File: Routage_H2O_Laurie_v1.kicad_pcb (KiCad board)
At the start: 2 copper layers, 110 x 100 mm, 54 parts, among them J2 Conn_01x02, J3 Conn_01x03, Q1 2N2907, Q10 TIP32, Q11 BD138, Q12 TIP31, Q13 2N2222, Q2 2N2907, Q3 2N2907, Q4 2N2222, Q5 2N2222, Q6 2N2907, Q7 2N2907, Q8 BD139, Q9 BD139, U1 Relay_1CT, U2 Jack_Mono

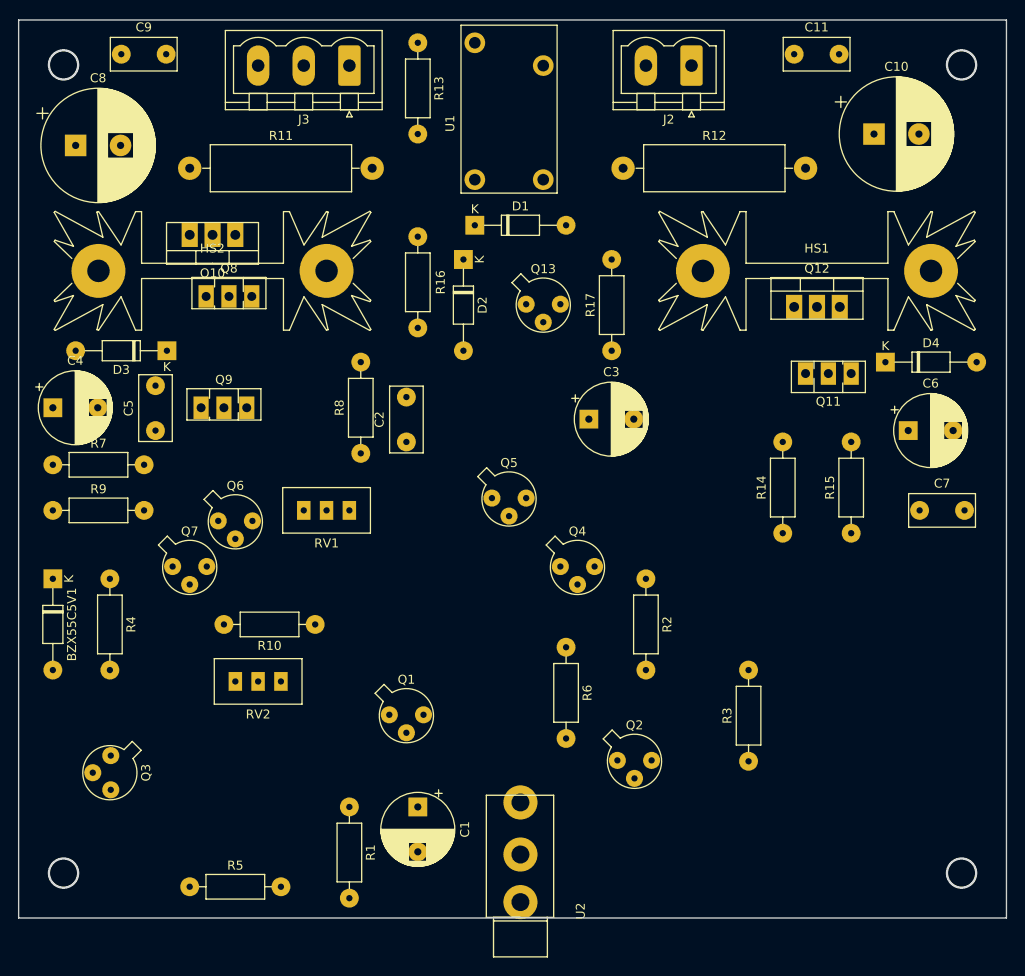
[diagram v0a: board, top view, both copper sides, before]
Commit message: Routagefinal
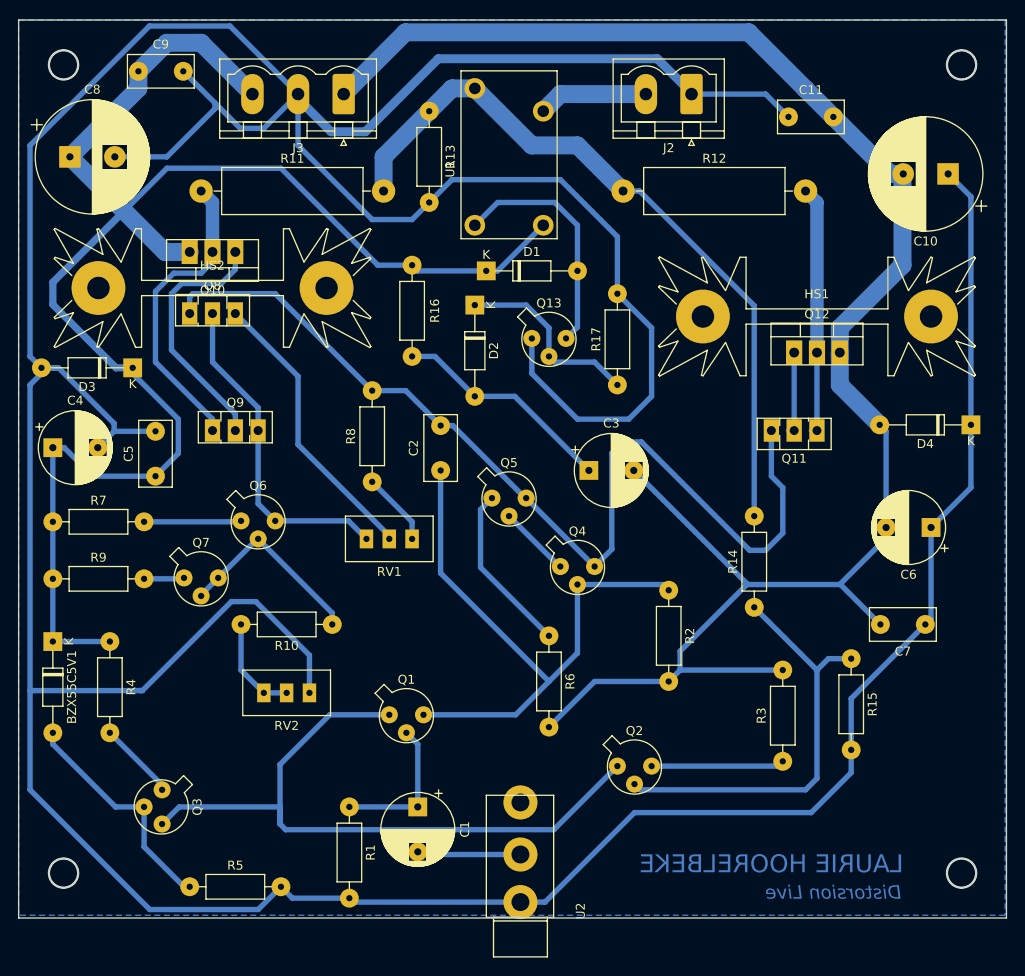
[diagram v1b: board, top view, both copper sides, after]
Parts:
- moved R15 14.0 mm to (181.6, 96.5), turned to 270 degrees
- moved C7 12.7 mm to (189.9, 92.7), turned to 180 degrees
- moved D4 11.8 mm to (194.9, 70.5), turned to 180 degrees
- moved C6 11.1 mm to (190.5, 81.9), turned to 180 degrees
- moved C10 9.38 mm to (192.4, 42.5), turned to 180 degrees
- moved R14 8.84 mm to (170.8, 90.8)
- moved R13 7.73 mm to (134.6, 35.6)
- moved RV1 7.67 mm to (127.6, 83.2)
- moved R9 7.62 mm to (92.7, 87.6)
- moved Q11 7.41 mm to (177.8, 71.1)
- moved C11 7.01 mm to (174.6, 36.2)
- moved BZX55C5V1 6.98 mm to (92.7, 94.6)
- moved R4 6.98 mm to (99.1, 94.6)
- moved Q3 6.87 mm to (104.8, 111.8)
- moved R7 6.35 mm to (92.7, 81.3)
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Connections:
- J2 pad 1: Net-(J2-Pad1) -> GND
- J2 pad 2: GND -> Net-(J2-Pad1)
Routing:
- net GND: track 0.00 -> 534.4 mm
- net -12V: track 0.00 -> 200.6 mm
- net +12V: track 0.00 -> 183.7 mm
- net Net-(C2-Pad2): track 0.00 -> 110.4 mm
- net Net-(R11-Pad2): track 0.00 -> 81.7 mm
- net Net-(Q1-Pad1): track 0.00 -> 77.7 mm
- net Net-(C2-Pad1): track 0.00 -> 66.5 mm
- net Net-(Q2-Pad2): track 0.00 -> 48.3 mm
- net Net-(Q6-Pad3): track 0.00 -> 37.0 mm
- net Net-(Q10-Pad2): track 0.00 -> 34.4 mm
- net Net-(Q8-Pad3): track 0.00 -> 32.2 mm
- net Net-(Q10-Pad1): track 0.00 -> 28.4 mm
- net Net-(Q11-Pad1): track 0.00 -> 28.1 mm
- net Net-(D1-Pad2): track 0.00 -> 26.7 mm
- net Net-(BZX55C5V1-Pad2): track 0.00 -> 25.7 mm
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- added copper zone on B.Cu, net GND
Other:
- board text added: "Distorsion Live"
- board text added: "LAURIE HOORELBEKE"
